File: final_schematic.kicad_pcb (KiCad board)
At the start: 2 copper layers, 54.7 x 60.6 mm, 56 parts, among them J1 Battery Babysitter, J2 BB_SYSOFF, J4 OLED Qwiic, J5 Programmer, J8 GPS_COAX, SW1 SW_Push_SESS, SW2 SW_Push_RADIO, SW3 SW_Push_RST, U1 STM32L476VGTx, U2 MTK3339, U3 RFM95W-868S2, U4 BNO055, U5 LT1129-3.3_SO8, U6 TC2014-3.3VxCTTR

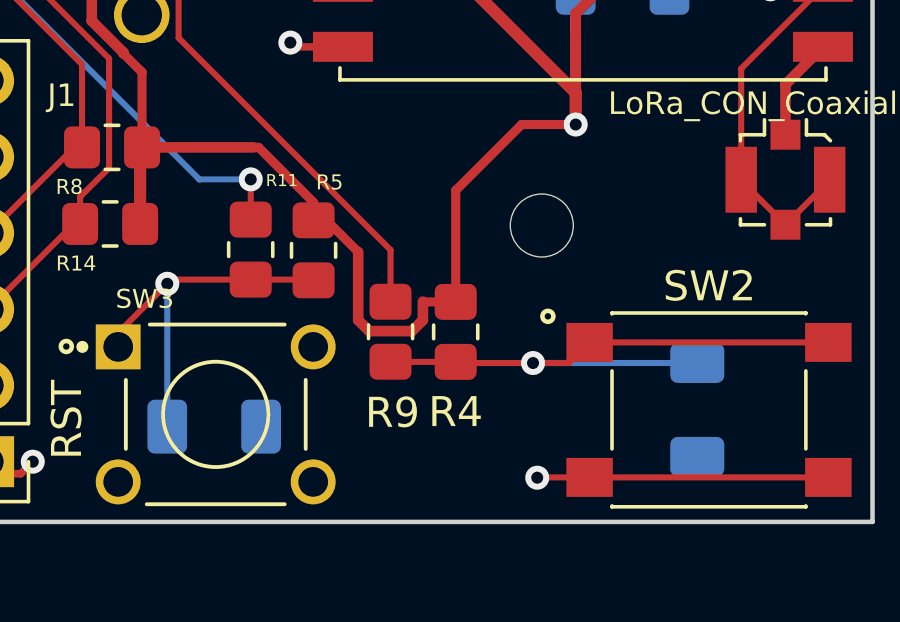
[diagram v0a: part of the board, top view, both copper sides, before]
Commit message: routing minimization peer review
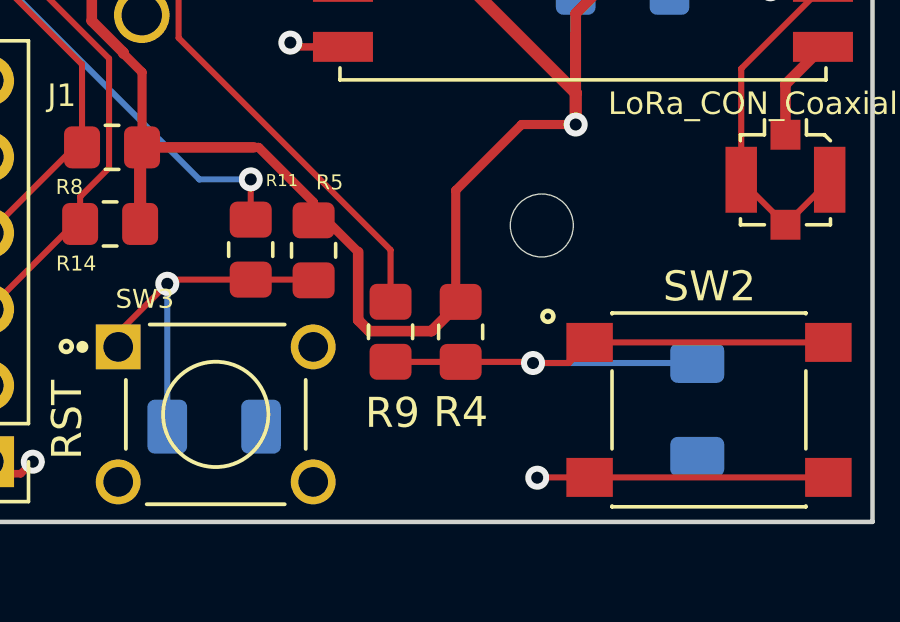
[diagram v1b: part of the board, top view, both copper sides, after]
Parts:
- moved R4 0.17 mm to (138.3, 99.6)
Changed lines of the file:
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@@
     (thickness 1.6)
     (drawings 51)
-    (tracks 573)
+    (tracks 572)
     (zones 0)
     (modules 56)
@@
   )
   (module Resistor_SMD:R_0805_2012Metric_Pad1.20x1.40mm_HandSolder (layer F.Cu)
-    (at 138.0998 99.5586 270)
+    (at 138.2649 99.5586 270)
     (descr "Resistor SMD 0805 (2012 Metric), square (rectangular) end terminal, IPC_7351 nominal with elongated pad for handsoldering. (Body size source: IPC-SM-782 page 72, https://www.pcb-3d.com/wordpress/wp-content/uploads/ipc-sm-782a_amendment_1_and_2.pdf), generated with kicad-footprint-generator")
     (tags "resistor handsolder")
@@
   (segment (start 140.6536 100.5724) (end 140.6775 100.5963) (width 0.2032) (layer F.Cu) (net 3))
   (segment (start 138.1375 100.5963) (end 138.0998 100.5586) (width 0.2032) (layer F.Cu) (net 3))
-  (segment (start 140.6775 100.5963) (end 138.1375 100.5963) (width 0.2032) (layer F.Cu) (net 3))
   (segment (start 135.9314 100.5586) (end 135.9281 100.5553) (width 0.2032) (layer F.Cu) (net 3))
   (segment (start 138.0998 100.5586) (end 135.9314 100.5586) (width 0.2032) (layer F.Cu) (net 3))
+  (segment (start 140.6398 100.5586) (end 140.6775 100.5963) (width 0.2032) (layer F.Cu) (net 3))
+  (segment (start 138.2649 100.5586) (end 140.6398 100.5586) (width 0.2032) (layer F.Cu) (net 3))
   (segment (start 128.4855 97.9547) (end 128.4855 97.9547) (width 0.25) (layer B.Cu) (net 4))
   (via (at 128.4855 97.9547) (size 0.8) (drill 0.4) (layers F.Cu B.Cu) (net 4))
@@
   (segment (start 111.6584 70.1929) (end 111.9251 70.1929) (width 0.6096) (layer B.Cu) (net 5))
   (segment (start 142.0999 92.6469) (end 140.2965 92.6469) (width 0.3048) (layer F.Cu) (net 5))
-  (segment (start 138.0998 94.8436) (end 138.0998 98.5586) (width 0.3048) (layer F.Cu) (net 5))
   (segment (start 140.2965 92.6469) (end 138.0998 94.8436) (width 0.3048) (layer F.Cu) (net 5))
   (segment (start 127.5809 93.472) (end 127.6444 93.4085) (width 0.4064) (layer F.Cu) (net 5))
   (segment (start 127.5809 95.9612) (end 127.5809 93.472) (width 0.4064) (layer F.Cu) (net 5))
-  (segment (start 136.63815 99.53311) (end 137.00591 99.16535) (width 0.3556) (layer F.Cu) (net 5))
-  (segment (start 135.21805 99.53311) (end 136.63815 99.53311) (width 0.3556) (layer F.Cu) (net 5))
-  (segment (start 134.85029 99.16535) (end 135.21805 99.53311) (width 0.3556) (layer F.Cu) (net 5))
-  (segment (start 134.85029 96.895438) (end 134.85029 99.16535) (width 0.3556) (layer F.Cu) (net 5))
   (segment (start 127.6444 93.4085) (end 131.363352 93.4085) (width 0.3556) (layer F.Cu) (net 5))
   (segment (start 127.6444 90.903262) (end 127.6444 93.4085) (width 0.3048) (layer F.Cu) (net 5))
@@
   (segment (start 133.3627 95.2408) (end 131.5304 93.4085) (width 0.3048) (layer F.Cu) (net 5))
   (segment (start 133.3627 95.8408) (end 133.3627 95.2408) (width 0.3048) (layer F.Cu) (net 5))
-  (segment (start 137.0142 98.5586) (end 137.00591 98.55031) (width 0.3048) (layer F.Cu) (net 5))
-  (segment (start 138.0998 98.5586) (end 137.0142 98.5586) (width 0.3048) (layer F.Cu) (net 5))
-  (segment (start 137.00591 99.16535) (end 137.00591 98.55031) (width 0.3556) (layer F.Cu) (net 5))
   (segment (start 143.3296 67.0586) (end 143.5608 66.8274) (width 0.254) (layer F.Cu) (net 5))
   (segment (start 142.0991 67.0586) (end 143.3296 67.0586) (width 0.254) (layer F.Cu) (net 5))
@@
   (segment (start 125.7596 85.5133) (end 125.9078 85.6615) (width 0.254) (layer F.Cu) (net 5))
   (segment (start 125.7596 84.129) (end 125.7596 85.5133) (width 0.254) (layer F.Cu) (net 5))
+  (segment (start 137.29039 99.53311) (end 138.2649 98.5586) (width 0.3556) (layer F.Cu) (net 5))
+  (segment (start 134.85029 99.16535) (end 135.21805 99.53311) (width 0.3556) (layer F.Cu) (net 5))
+  (segment (start 135.21805 99.53311) (end 137.29039 99.53311) (width 0.3556) (layer F.Cu) (net 5))
+  (segment (start 134.85029 96.895438) (end 134.85029 99.16535) (width 0.3556) (layer F.Cu) (net 5))
+  (segment (start 138.0998 98.3935) (end 138.2649 98.5586) (width 0.3048) (layer F.Cu) (net 5))
+  (segment (start 138.0998 94.8436) (end 138.0998 98.3935) (width 0.3048) (layer F.Cu) (net 5))
   (segment (start 135.9567 68.0586) (end 135.89 67.9919) (width 0.2032) (layer F.Cu) (net 6))
   (segment (start 138.7741 68.0586) (end 135.9567 68.0586) (width 0.2032) (layer F.Cu) (net 6))
